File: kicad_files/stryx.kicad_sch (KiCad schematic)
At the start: 28 parts, among them J1 Screw_Terminal_M1, J1 USB_B_Micro, J2 Screw_Terminal_M2, J3 Screw_Terminal_Power, SW1 SW_SPDT, U1 LM317_TO-220, U2 NUCLEO-L432KC, U3 TB6612FNG-Module, U4 HC-SR04, U5 NRF24L01_Breakout

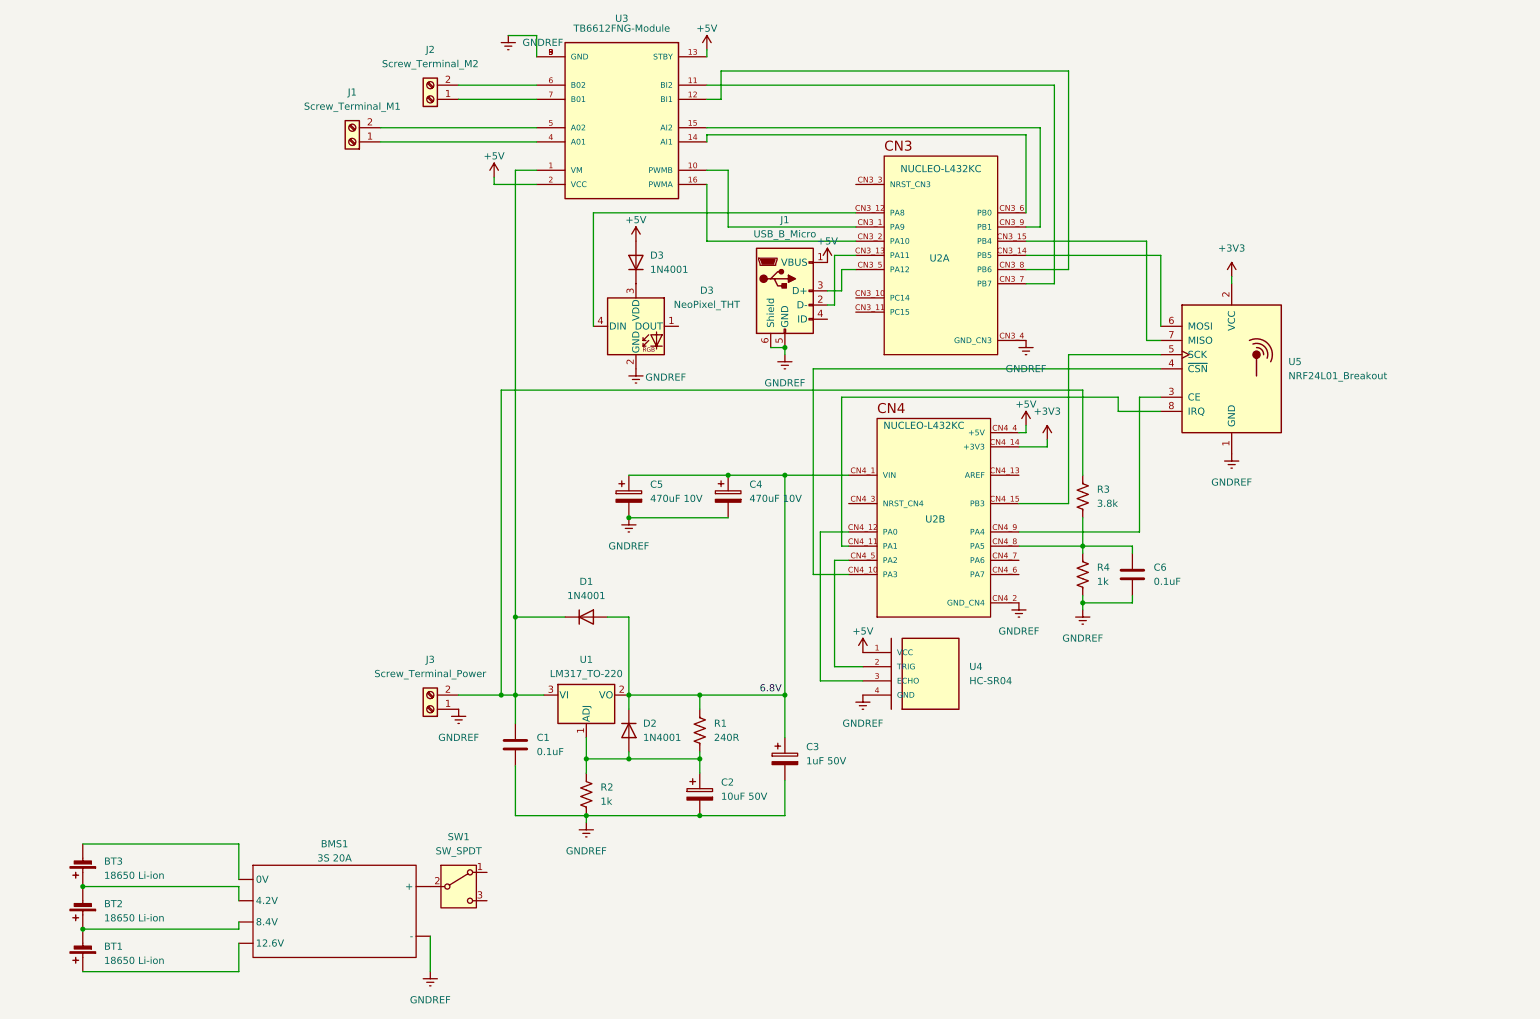
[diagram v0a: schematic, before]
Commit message: Updated kicad schematic
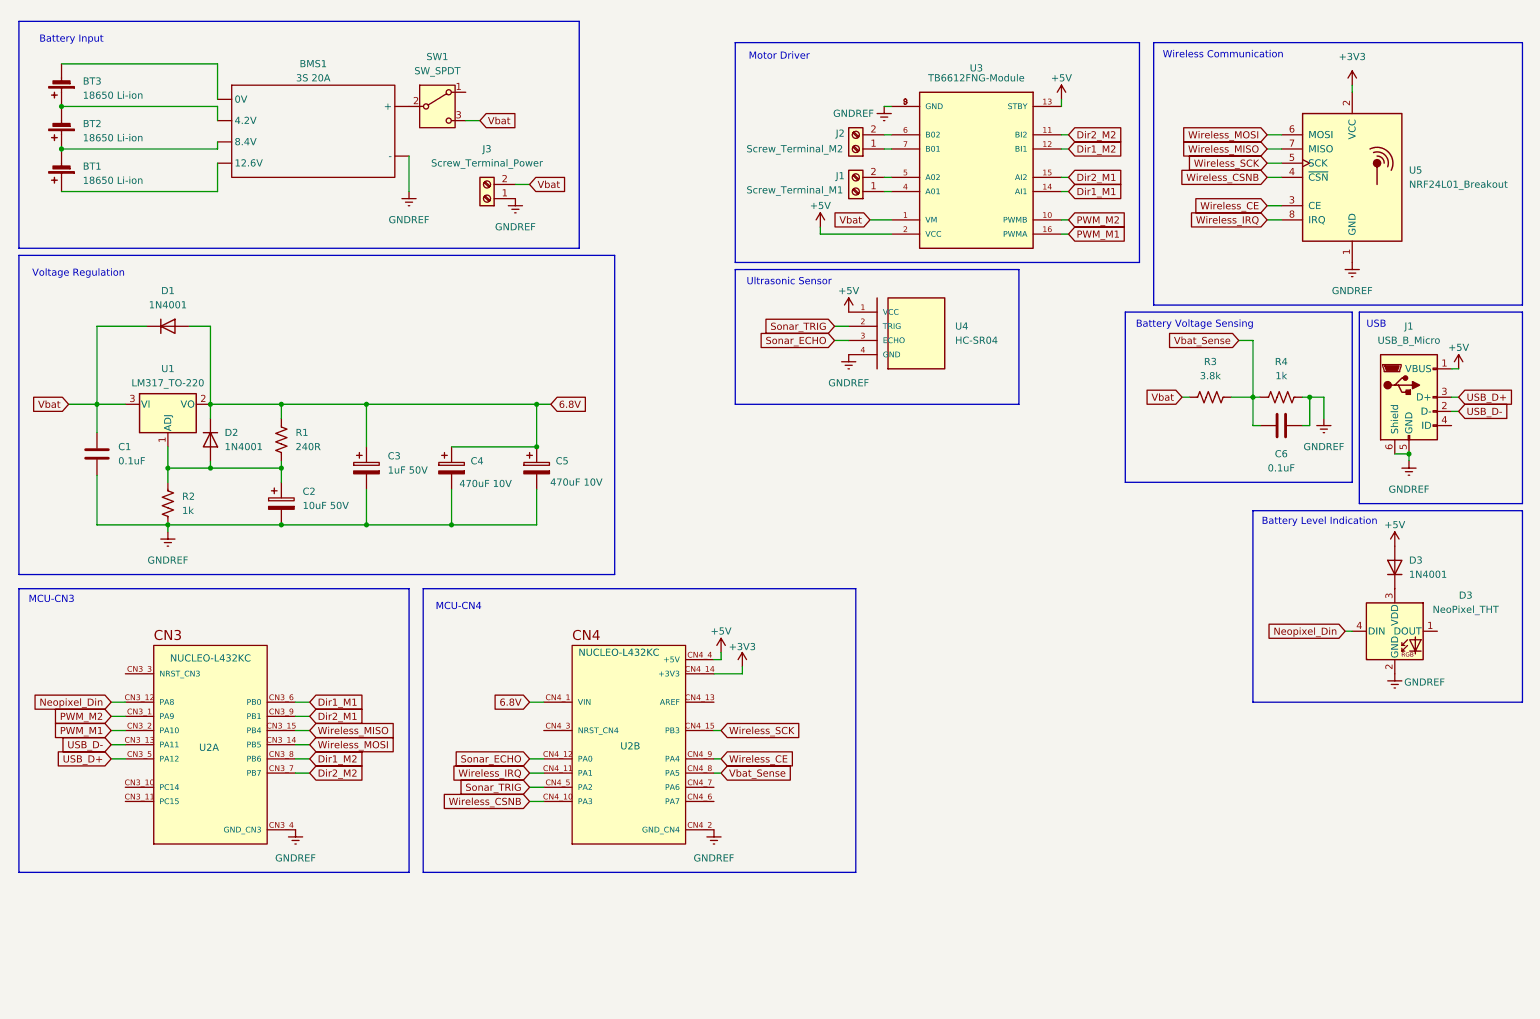
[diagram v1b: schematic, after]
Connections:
- net GNDREF: now also C6.1; no longer C6.2
- net Neopixel_Din: now reaches D3.4 (DIN), U2.CN3_12 (PA8)
- net 6.8V: now reaches C3.1, C4.1, C5.1, D1.2 (A), D2.1 (K), R1.1, U1.2 (VO), U2.CN4_1 (VIN)
- net Vbat_Sense: now reaches R3.2, R4.1, U2.CN4_8 (PA5)
- net Vbat_Sense: now also C6.2; no longer C6.1
- net Vbat: now reaches C1.2, D1.1 (K), J3.2 (Pin_2), R3.1, U1.3 (VI), U3.1 (VM)
- net Vbat: now also SW1.3 (C)
- net PWM_M2: now reaches U2.CN3_1 (PA9), U3.10 (PWMB)
- net Dir2_M2: now reaches U2.CN3_7 (PB7), U3.11 (BI2)
- net Dir1_M2: now reaches U2.CN3_8 (PB6), U3.12 (BI1)
- net Dir1_M1: now reaches U2.CN3_6 (PB0), U3.14 (AI1)
- net Dir2_M1: now reaches U2.CN3_9 (PB1), U3.15 (AI2)
- net PWM_M1: now reaches U2.CN3_2 (PA10), U3.16 (PWMA)
- net Sonar_TRIG: now reaches U2.CN4_5 (PA2), U4.2 (TRIG)
- net Sonar_ECHO: now reaches U2.CN4_12 (PA0), U4.3 (ECHO)
- net USB_D-: now reaches J1.2 (D-), U2.CN3_13 (PA11)
- net USB_D+: now reaches J1.3 (D+), U2.CN3_5 (PA12)
- net Wireless_MOSI: now reaches U2.CN3_14 (PB5), U5.6 (MOSI)
- net Wireless_MISO: now reaches U2.CN3_15 (PB4), U5.7 (MISO)
- net Wireless_CSNB: now reaches U2.CN4_10 (PA3), U5.4 (~{CSN})
- net Wireless_IRQ: now reaches U2.CN4_11 (PA1), U5.8 (IRQ)
- net Wireless_SCK: now reaches U2.CN4_15 (PB3), U5.5 (SCK)
- net Wireless_CE: now reaches U2.CN4_9 (PA4), U5.3 (CE)
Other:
- note added: "Battery Input"
- note added: "Battery Level Indication"
- note added: "Battery Voltage Sensing"
- note added: "MCU-CN3"
- note added: "MCU-CN4"
- note added: "Motor Driver"
- note added: "USB"
- note added: "Ultrasonic Sensor"
- note added: "Voltage Regulation"
- note added: "Wireless Communication"
- note removed: "6.8V"
- moved on the sheet: BMS1, BT1, BT2, BT3, C1, C2, C3, C4, C5, C6, D1, D2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
